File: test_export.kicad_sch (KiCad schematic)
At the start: 2 parts, among them U1 TestMCU

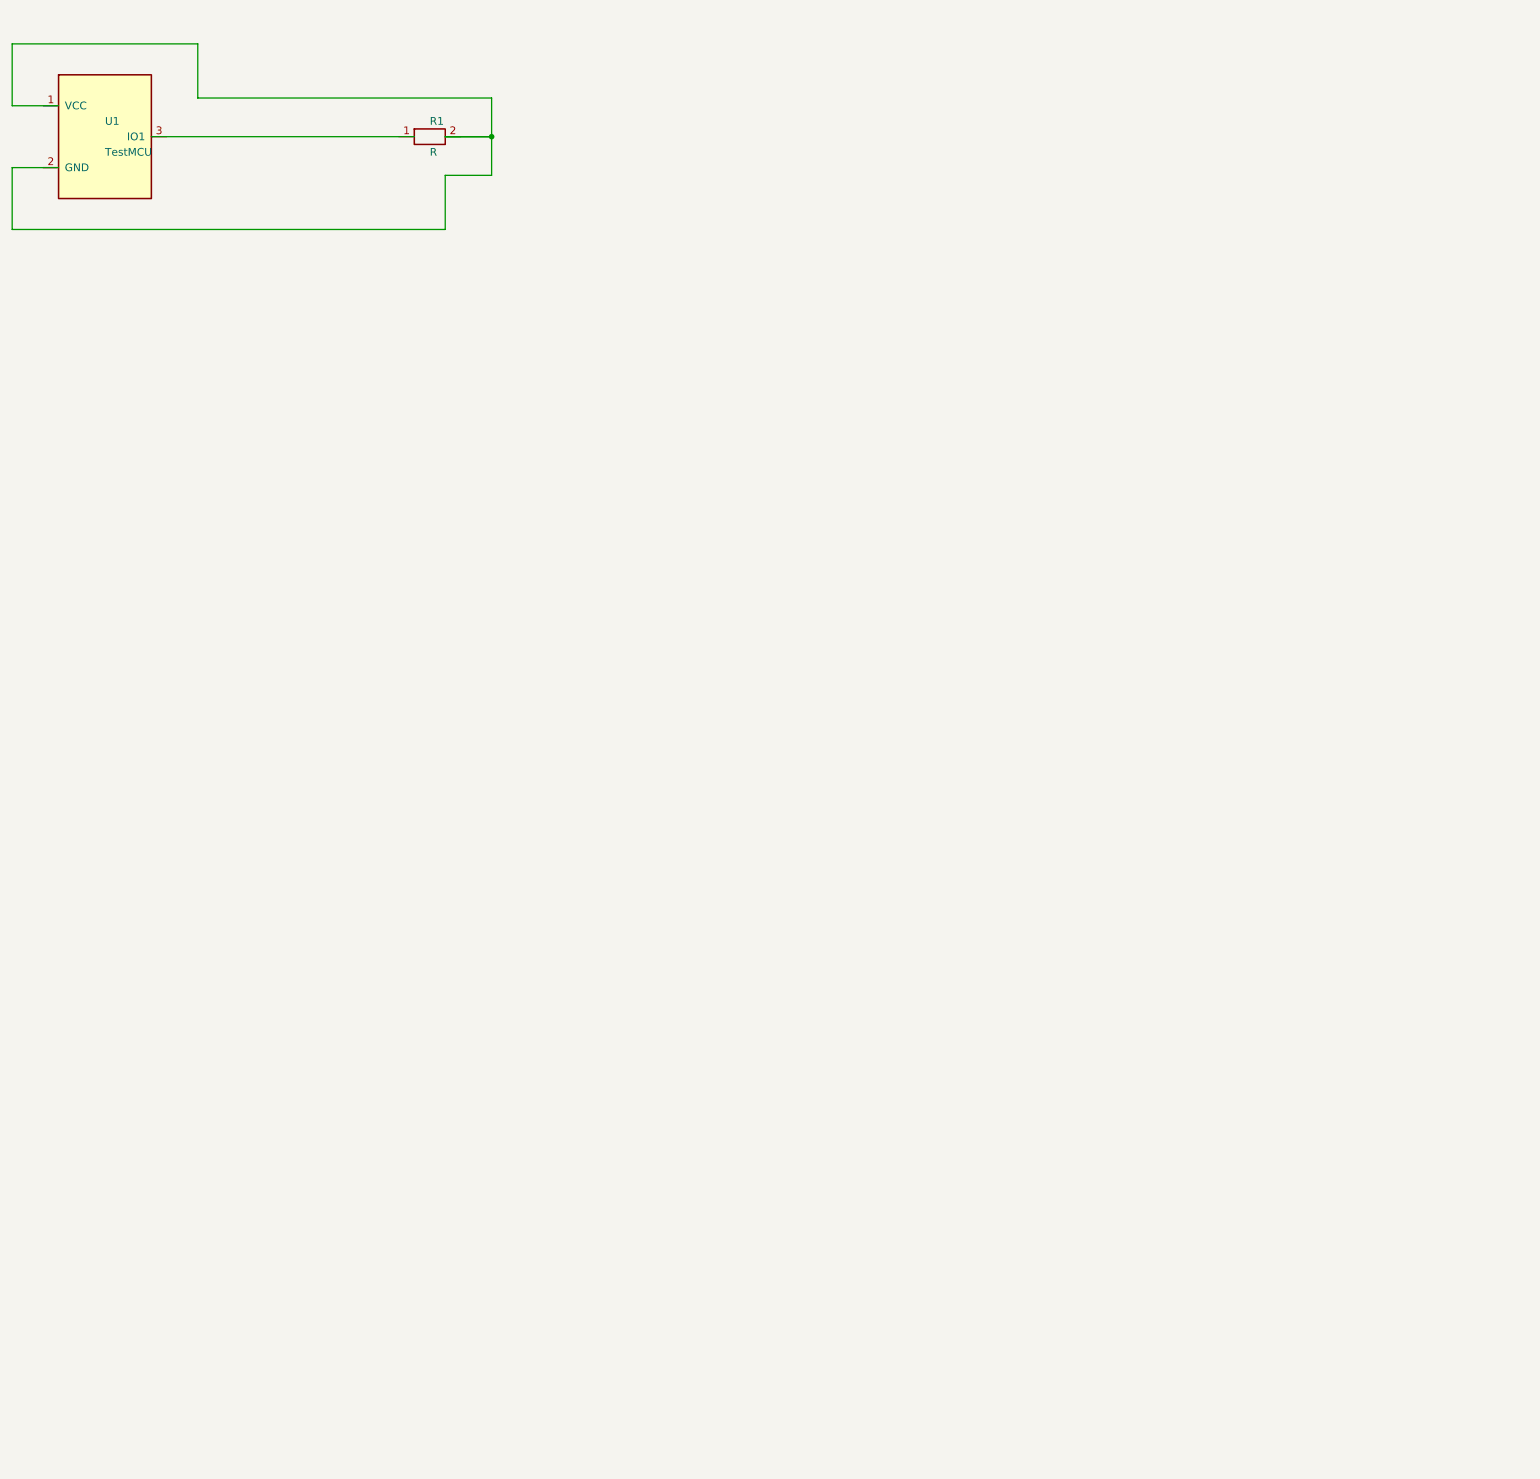
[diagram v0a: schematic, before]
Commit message: feat: merge main into feature/layout-routing-engine - UI redesign, routing fixes, hallucination resolver, support components
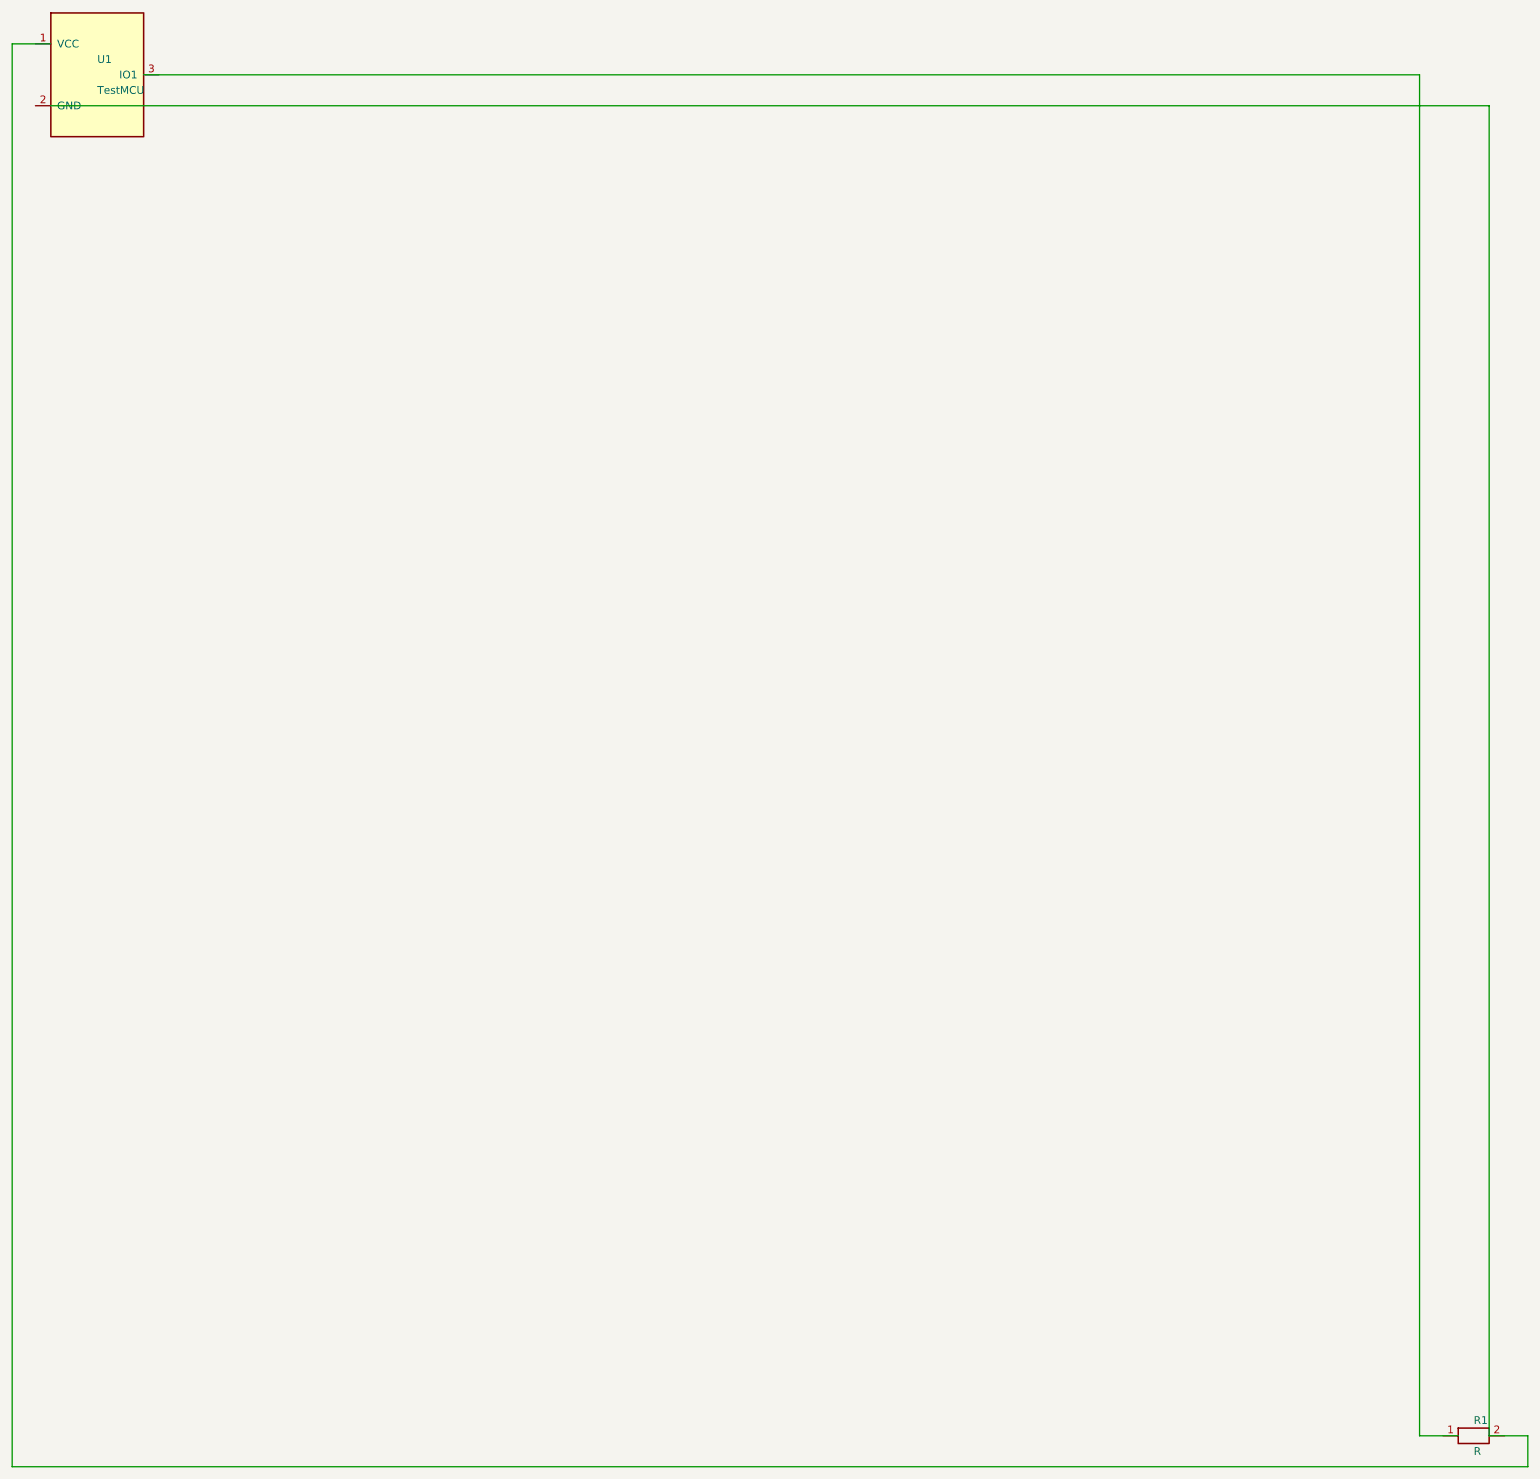
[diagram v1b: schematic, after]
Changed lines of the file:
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@@
 (kicad_sch (version 20231120) (generator "circuitbot") (generator_version "1.0")
   (paper "A3")
-  (symbol (lib_id "MCU_Module:TestMCU") (at 66.04 66.04 0) (unit 1)
+  (symbol (lib_id "MCU_Module:TestMCU") (at 64.77 55.88 0) (unit 1)
     (in_bom yes) (on_board yes) (dnp no)
-    (property "Reference" "U1" (at 66.04 63.5 0)
+    (property "Reference" "U1" (at 64.77 53.34 0)
       (effects (font (size 1.27 1.27)) (justify left))
     )
-    (property "Value" "TestMCU" (at 66.04 68.58 0)
+    (property "Value" "TestMCU" (at 64.77 58.42 0)
       (effects (font (size 1.27 1.27)) (justify left))
     )
-    (property "Footprint" "" (at 66.04 66.04 0)
+    (property "Footprint" "" (at 64.77 55.88 0)
       (effects (font (size 1.27 1.27)) hide)
     )
-    (property "Datasheet" "" (at 66.04 66.04 0)
+    (property "Datasheet" "" (at 64.77 55.88 0)
       (effects (font (size 1.27 1.27)) hide)
     )
@@
     (instances
       (project "circuitbot"
-        (path "/887a8ce8-c090-460f-8dcc-88c952b0be6d" (reference "U1") (unit 1))
+        (path "/0c6ad7ac-714a-4d90-9f20-ea719fcfd868" (reference "U1") (unit 1))
       )
     )
   )
-  (symbol (lib_id "Device:R") (at 119.38 66.04 0) (unit 1)
+  (symbol (lib_id "Device:R") (at 290.83 279.4 0) (unit 1)
     (in_bom yes) (on_board yes) (dnp no)
-    (property "Reference" "R1" (at 119.38 63.5 0)
+    (property "Reference" "R1" (at 290.83 276.86 0)
       (effects (font (size 1.27 1.27)) (justify left))
     )
-    (property "Value" "R" (at 119.38 68.58 0)
+    (property "Value" "R" (at 290.83 281.94 0)
       (effects (font (size 1.27 1.27)) (justify left))
     )
-    (property "Footprint" "" (at 119.38 66.04 0)
+    (property "Footprint" "" (at 290.83 279.4 0)
       (effects (font (size 1.27 1.27)) hide)
     )
-    (property "Datasheet" "" (at 119.38 66.04 0)
+    (property "Datasheet" "" (at 290.83 279.4 0)
       (effects (font (size 1.27 1.27)) hide)
     )
@@
     (instances
       (project "circuitbot"
-        (path "/887a8ce8-c090-460f-8dcc-88c952b0be6d" (reference "R1") (unit 1))
+        (path "/0c6ad7ac-714a-4d90-9f20-ea719fcfd868" (reference "R1") (unit 1))
       )
     )
   )
-  (wire (pts (xy 73.66 66.04) (xy 116.84 66.04))
+  (wire (pts (xy 72.39 55.88) (xy 281.94 55.88))
     (stroke (width 0) (type default))
   )
-  (wire (pts (xy 58.42 60.96) (xy 50.8 60.96))
+  (wire (pts (xy 281.94 55.88) (xy 281.94 279.4))
     (stroke (width 0) (type default))
   )
-  (wire (pts (xy 50.8 60.96) (xy 50.8 50.8))
+  (wire (pts (xy 281.94 279.4) (xy 288.29 279.4))
     (stroke (width 0) (type default))
   )
-  (wire (pts (xy 50.8 50.8) (xy 81.28 50.8))
+  (wire (pts (xy 57.15 50.8) (xy 50.8 50.8))
     (stroke (width 0) (type default))
   )
-  (wire (pts (xy 81.28 50.8) (xy 81.28 59.69))
+  (wire (pts (xy 50.8 50.8) (xy 50.8 284.48))
     (stroke (width 0) (type default))
   )
-  (wire (pts (xy 81.28 59.69) (xy 129.54 59.69))
+  (wire (pts (xy 50.8 284.48) (xy 299.72 284.48))
     (stroke (width 0) (type default))
   )
-  (wire (pts (xy 129.54 59.69) (xy 129.54 66.04))
+  (wire (pts (xy 299.72 284.48) (xy 299.72 279.4))
     (stroke (width 0) (type default))
   )
-  (wire (pts (xy 129.54 66.04) (xy 121.92 66.04))
+  (wire (pts (xy 299.72 279.4) (xy 293.37 279.4))
     (stroke (width 0) (type default))
   )
-  (wire (pts (xy 58.42 71.12) (xy 50.8 71.12))
+  (wire (pts (xy 57.15 60.96) (xy 293.37 60.96))
     (stroke (width 0) (type default))
   )
-  (wire (pts (xy 50.8 71.12) (xy 50.8 81.28))
+  (wire (pts (xy 293.37 60.96) (xy 293.37 279.4))
     (stroke (width 0) (type default))
   )
-  (wire (pts (xy 50.8 81.28) (xy 121.92 81.28))
-    (stroke (width 0) (type default))
-  )
-  (wire (pts (xy 121.92 81.28) (xy 121.92 72.39))
-    (stroke (width 0) (type default))
-  )
-  (wire (pts (xy 121.92 72.39) (xy 129.54 72.39))
-    (stroke (width 0) (type default))
-  )
-  (wire (pts (xy 129.54 72.39) (xy 129.54 66.04))
-    (stroke (width 0) (type default))
-  )
-  (wire (pts (xy 129.54 66.04) (xy 121.92 66.04))
-    (stroke (width 0) (type default))
-  )
-  (junction (at 129.54 66.04) (diameter 0) (color 0 0 0 0)
-  )
   (sheet_instances (path "/" (page "1")))
